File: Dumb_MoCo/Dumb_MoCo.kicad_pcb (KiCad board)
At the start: 2 copper layers, 32.7 x 55.3 mm, 20 parts, among them U1 VNH7070AS

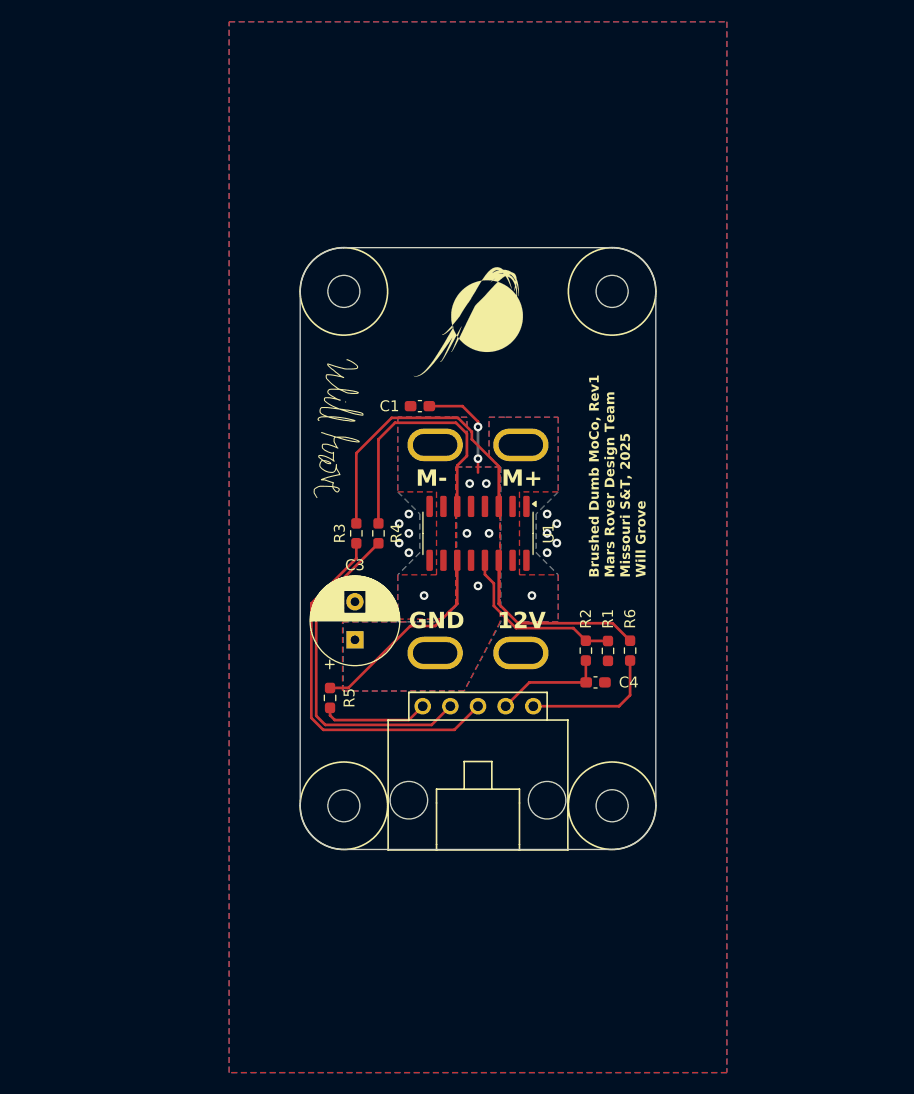
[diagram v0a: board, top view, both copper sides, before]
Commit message: Started on layout
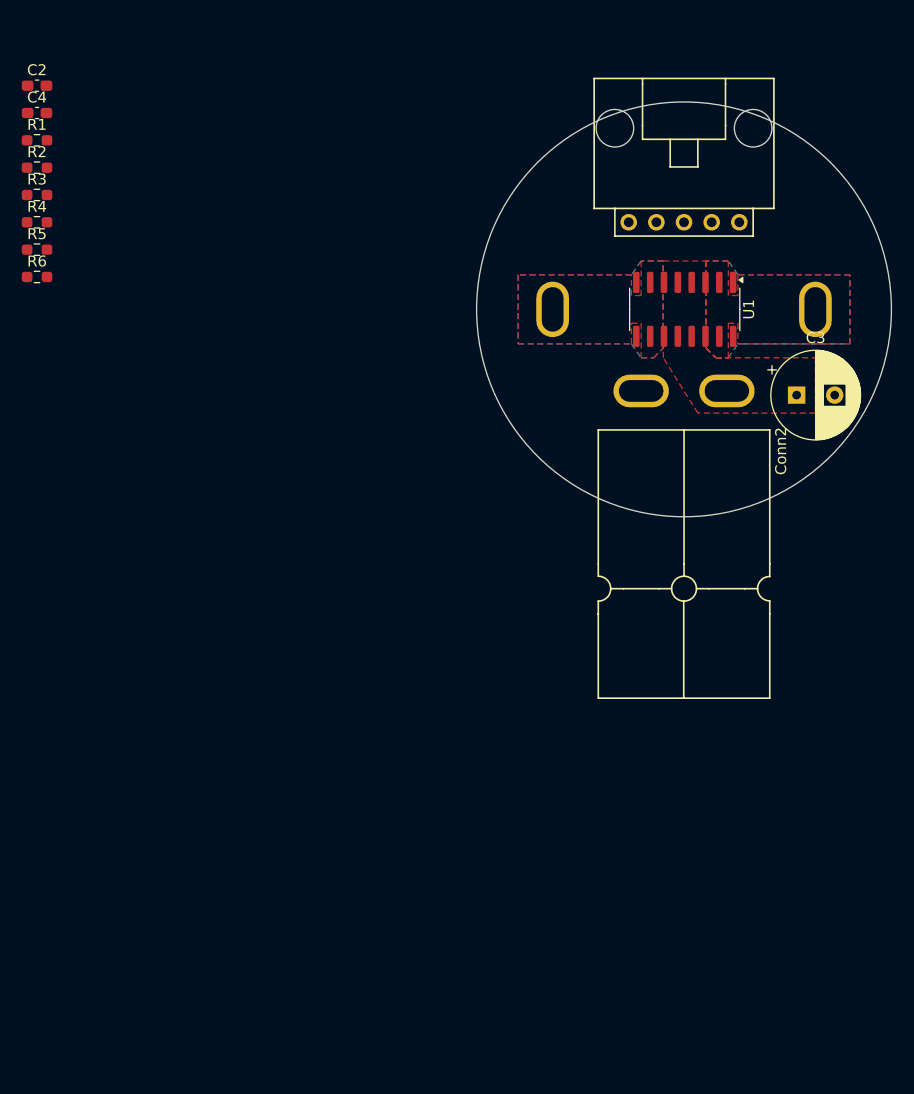
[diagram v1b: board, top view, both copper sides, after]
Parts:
- removed C1: 10uF, Capacitor_SMD:C_0603_1608Metric_Pad1.08x0.95mm_HandSolder
- removed G***: LOGO, MRDT_Silkscreens:0_MRDT_Logo_10mm
- removed G***: LOGO, Signatures:WillGroveSignatureMedium
- removed G***: LOGO, Signatures:ChamberUlt
- removed V1, V2, V3, V4: Via, MRDT_Drill_Holes:4_40_Hole
- added C2: 0.1uF, Capacitor_SMD:C_0603_1608Metric_Pad1.08x0.95mm_HandSolder, F.Cu at (94.2, 52.5)
- Conn1, Conn2: moved to F.Cu
- moved C4 73.3 mm to (94.2, 55.0), turned to 0 degrees
- moved R1 70.4 mm to (94.2, 57.5), turned to 0 degrees
- moved R2 67.1 mm to (94.2, 60.0), turned to 0 degrees
- moved R6 64.4 mm to (94.2, 70.0), turned to 0 degrees
- moved R5 49.2 mm to (94.2, 67.5), turned to 0 degrees
- moved C3 46.4 mm to (164.0, 80.9), turned to 0 degrees
- moved Conn3 45.3 mm to (148.6, 65.0), turned to 0 degrees
- moved R3 42.7 mm to (94.2, 62.5), turned to 0 degrees
- moved R4 42.4 mm to (94.2, 65.0), turned to 0 degrees
- moved U1 28.0 mm to (153.7, 73.0)
- moved Conn2 26.0 mm to (149.2, 80.1)
- moved Conn1 17.6 mm to (141.6, 72.4), turned to 0 degrees
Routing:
- net IN_A: track 34.4 -> 0.00 mm
- net IN_B: track 31.6 -> 0.00 mm
- net Net-(U1-IN_A): track 26.8 -> 0.00 mm
- net Net-(U1-IN_B): track 23.9 -> 0.00 mm
- net Net-(U1-PWM): track 18.9 -> 0.00 mm
- net Net-(U1-SEL): track 17.5 -> 0.00 mm
- net Net-(U1-CS): track 16.3 -> 0.00 mm
- net SEL: track 12.5 -> 0.00 mm
- net CS: track 10.3 -> 0.00 mm
- net PWM: track 9.90 -> 0.00 mm
- net +12V: track 9.74 -> 0.00 mm, vias 7 -> 0
- net GND: vias 10 -> 0
- net /M-: vias 1 -> 0
- net /M+: vias 1 -> 0
- removed copper zone on B.Cu, net +12V
- removed copper zone on B.Cu, net GND
- removed copper zone on F.Cu, net GND
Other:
- board size 32.7 x 55.3 mm -> 38.1 x 38.1 mm
- board text removed: "12V"
- board text removed: "Brushed Dumb MoCo, Rev1 Mars Rover Design Team Missouri S&T, 2025 Will Grove"
- board text removed: "GND"
- board text removed: "M+"
- board text removed: "M-"
